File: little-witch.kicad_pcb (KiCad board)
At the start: 4 copper layers, 65 x 30 mm, 56 parts, among them J1 GCT-USB4105, J2 TMJG0803HENL, J3 Conn_ARM_SWD_TagConnect_TC203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, J4 GCT-USB4105, J5 Conn_02x20_Odd_Even, J6 BOOT0_SEL, SW1 SW_Push, U1 CH32V307RCT6, U2 MXL86110C-AQB-R, Y1 SIT8008BI-73-33N-25.000000

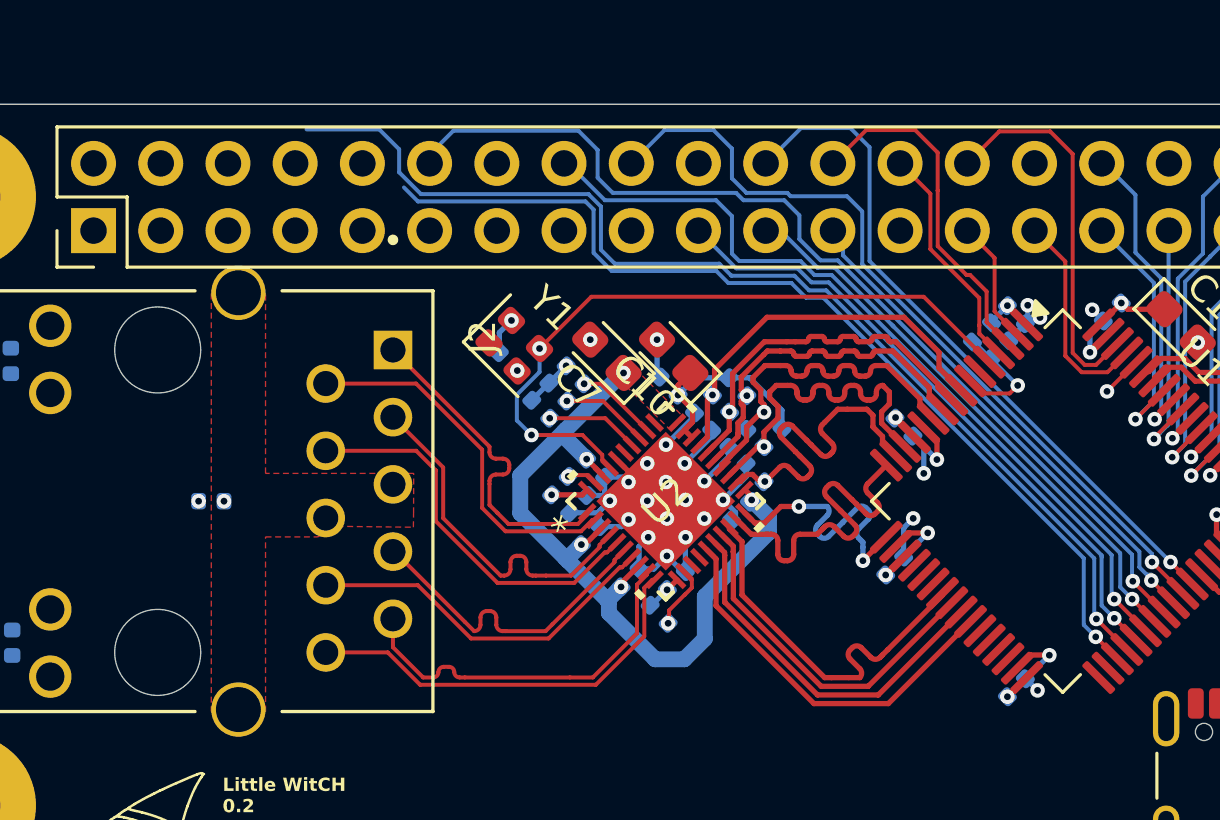
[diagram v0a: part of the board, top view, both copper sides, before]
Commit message: GPIO fully routed
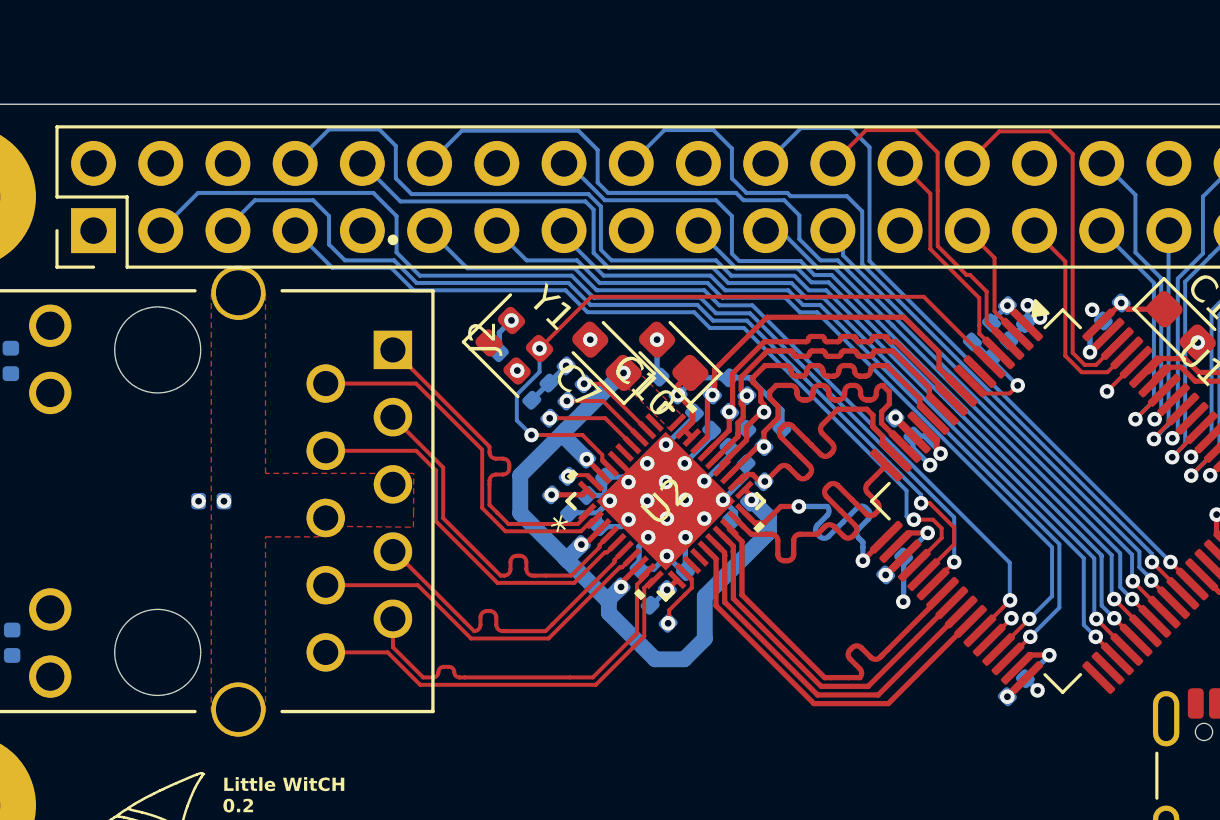
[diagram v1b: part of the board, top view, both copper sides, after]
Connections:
- J5 pad 11: unconnected-(J5-Pin_11-Pad11) -> /PB1
- J5 pad 13: unconnected-(J5-Pin_13-Pad13) -> /PB10
- J5 pad 15: unconnected-(J5-Pin_15-Pad15) -> /PB11
- J5 pad 3: unconnected-(J5-Pin_3-Pad3) -> /PA6
- J5 pad 5: unconnected-(J5-Pin_5-Pad5) -> /PA5
- J5 pad 7: unconnected-(J5-Pin_7-Pad7) -> /PA4
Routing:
- net /PA6: track 0.00 -> 39.3 mm, vias 0 -> 1
- net /PA5: track 0.00 -> 36.2 mm, vias 0 -> 1
- net /PA4: track 0.00 -> 31.5 mm, vias 0 -> 1
- net /PB10: track 0.00 -> 30.6 mm, vias 0 -> 1
- net /PB1: track 0.00 -> 30.2 mm, vias 0 -> 1
- net /PB11: track 0.00 -> 28.9 mm, vias 0 -> 1
- net /PB14: track 36.8 -> 38.7 mm
- net /PB2: track 0.00 -> 1.18 mm, vias 0 -> 1
- net /PB15: track 41.9 -> 43.1 mm
